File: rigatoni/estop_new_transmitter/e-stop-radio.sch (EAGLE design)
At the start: 71 parts, among them J2 AVR_SPI_PROG_3X2PTH, J3 UX60-MB-5S8, J4 5-1814832-1, Q1 MMUN2133LT1G, U1 ATMEGA32U4-AU, U2 MCP73831T-2ACI/OT, U3 TPS62203DBVR, U4 TPS61090RSAR, U5 RFM69HCW, U6 SN74ALVC164245DGGR, X1 TSX-3225 16.0000MF18X-AC0

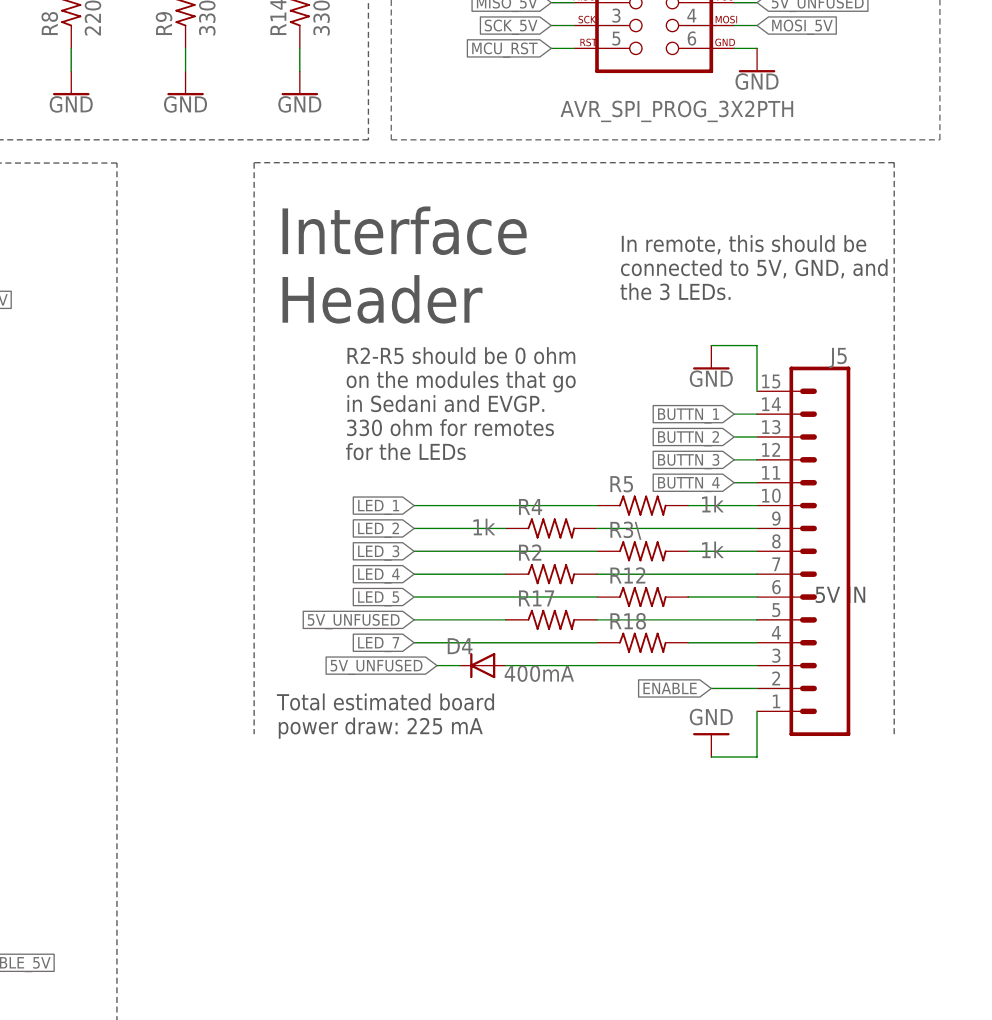
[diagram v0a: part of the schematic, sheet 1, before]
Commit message: Rough PCB Design Complete
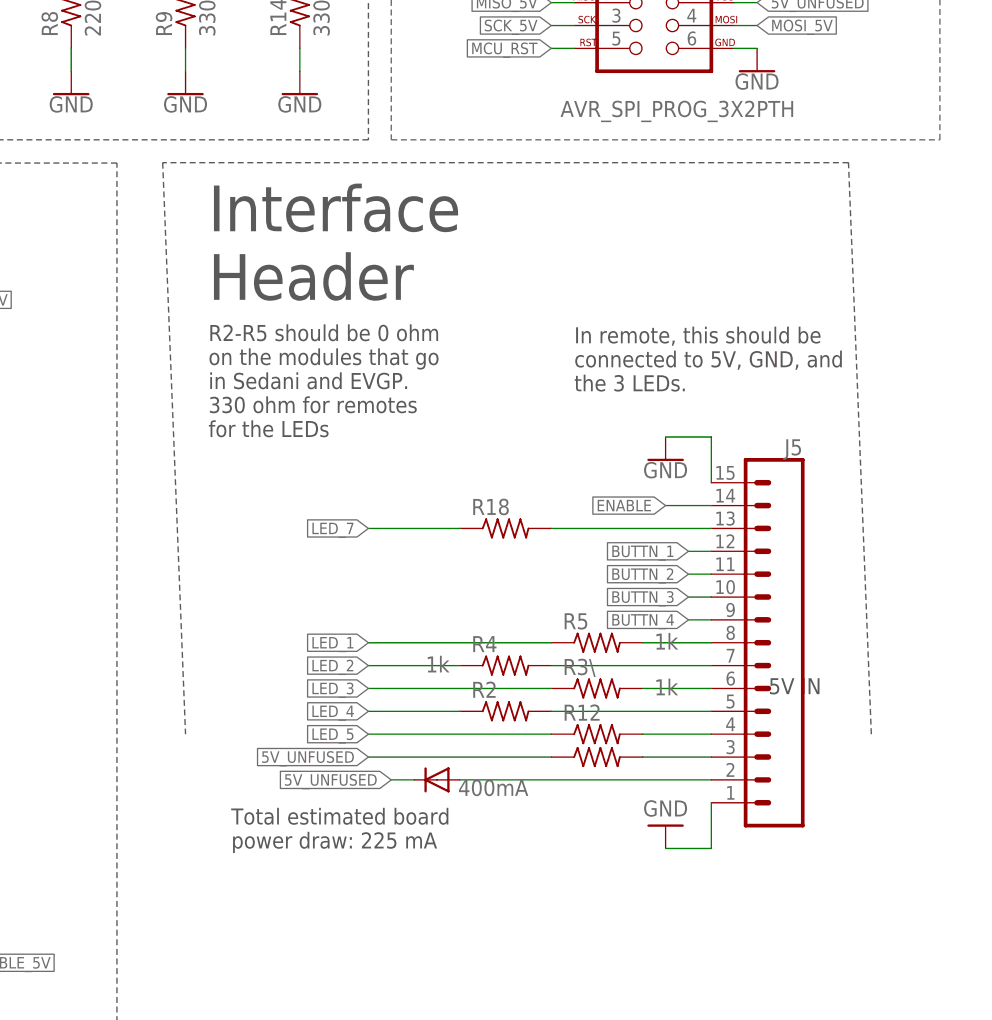
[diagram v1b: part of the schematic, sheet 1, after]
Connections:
- net BUTTN_1: now also J5.12; no longer J5.14
- net BUTTN_2: now also J5.11; no longer J5.13
- net BUTTN_3: now also J5.10; no longer J5.12
- net BUTTN_4: now also J5.9; no longer J5.11
- net DIO_4_R: now also J5.8; no longer J5.10
- net DIO_5_R: now also J5.7; no longer J5.9
- net DIO_6_R: now also J5.6; no longer J5.8
- net DIO_7_R: now also J5.5; no longer J5.7
- net DIO_7_R1: now also J5.4; no longer J5.6
- net DIO_7_R2: now also J5.3; no longer J5.5
- net DIO_7_R3: now also J5.13; no longer J5.4
- net ENABLE: now also J5.14; no longer J5.2
- net H4: now also J5.2; no longer J5.3
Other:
- moved on the sheet: J5, R12, R18, R2, R3\, R4, R5
